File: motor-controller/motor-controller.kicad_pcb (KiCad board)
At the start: 4 copper layers, 30.5 x 51.3 mm, 43 parts, among them J1 SCREW +, J2 SCREW -, J3 SCREW MOTOR A, J4 SCREW MOTOR B, J5 Conn_01x05, J6 Conn_01x03, Q1 EPC2206, Q2 EPC2206, Q3 EPC2206, Q4 EPC2206, U1 uP1966E, U2 uP1966E, U4 STM32G030F6P6TR, U5 NCP1117ST33T3G, U6 LM78M05

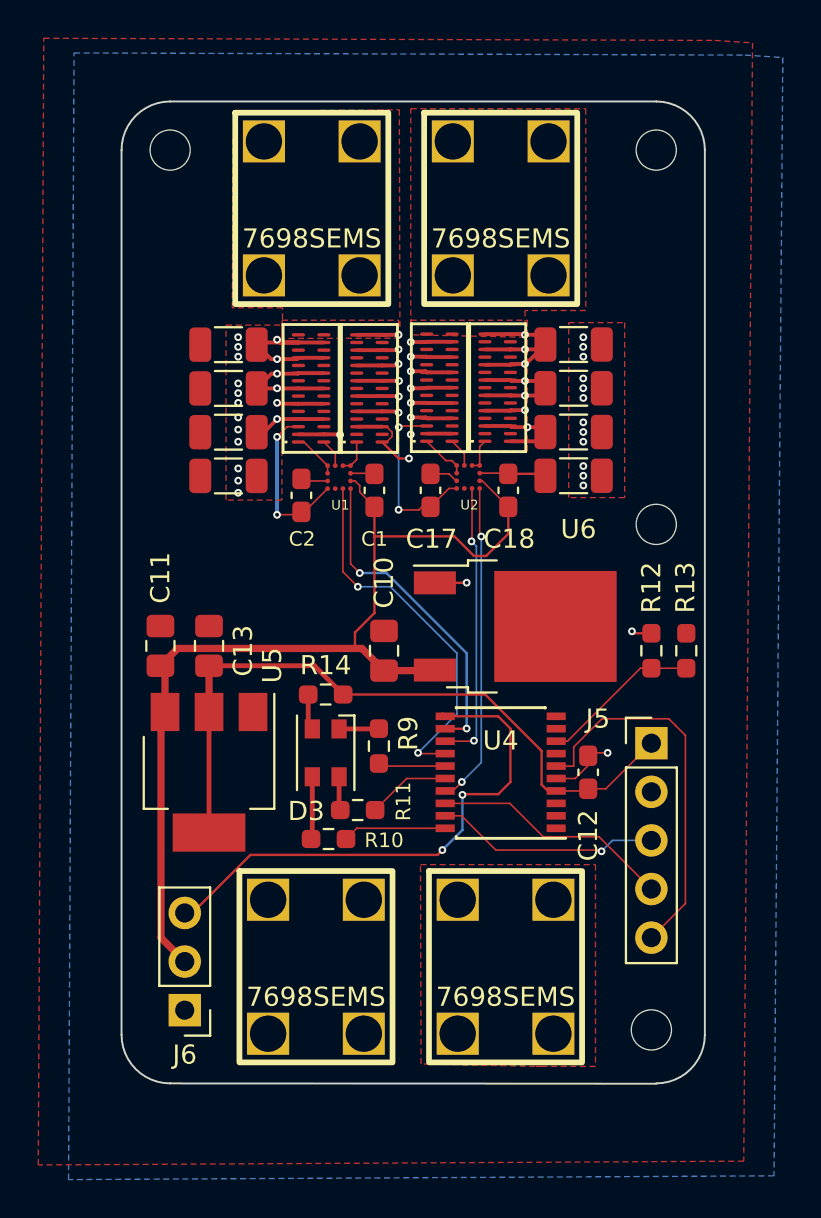
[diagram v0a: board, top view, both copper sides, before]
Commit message: Add in released stuff
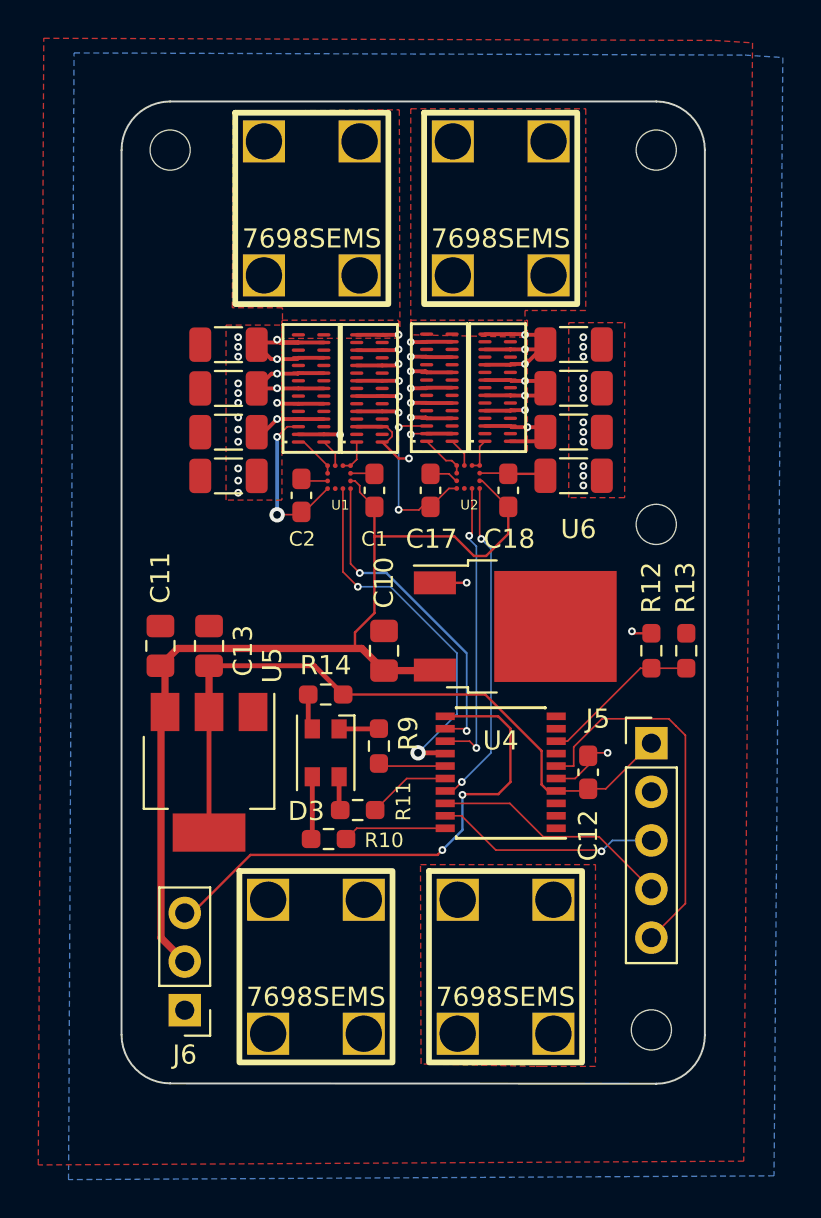
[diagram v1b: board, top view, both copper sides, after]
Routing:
- net VBUS: track 41.4 -> 42.3 mm
- net PWM_B_LOW: track 16.6 -> 17.3 mm
- net PWM_B_HIGH: track 15.0 -> 15.6 mm
